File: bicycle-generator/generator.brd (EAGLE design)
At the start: 100 x 80 mm, 62 parts, among them IC1 MC34063AD, K1 ARK500/2, K2 ARK500/2, K3 ARK500/2, K4 ARK500/2, K5 ARK500/2, K6 HEAT_NPN, K7 ARK500/2, K8 ARK500/2, Q1 IRF3704S, Q2 IRF3704S, T1 BC807, T2 BC807, X1 CV_LED, X2 PWR_LED, X3 5V_SW, X4 5V_LED, X5 5V_OUT

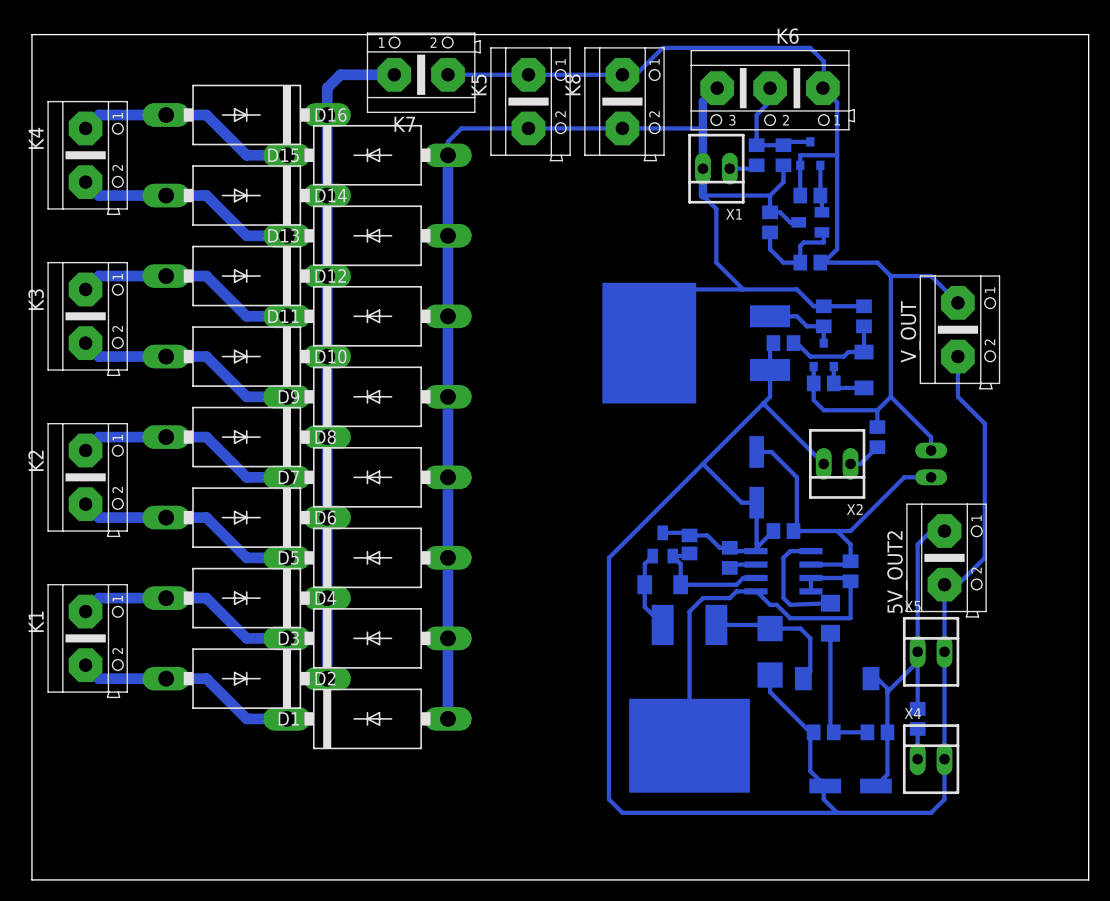
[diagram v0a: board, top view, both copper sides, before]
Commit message: Routed board.
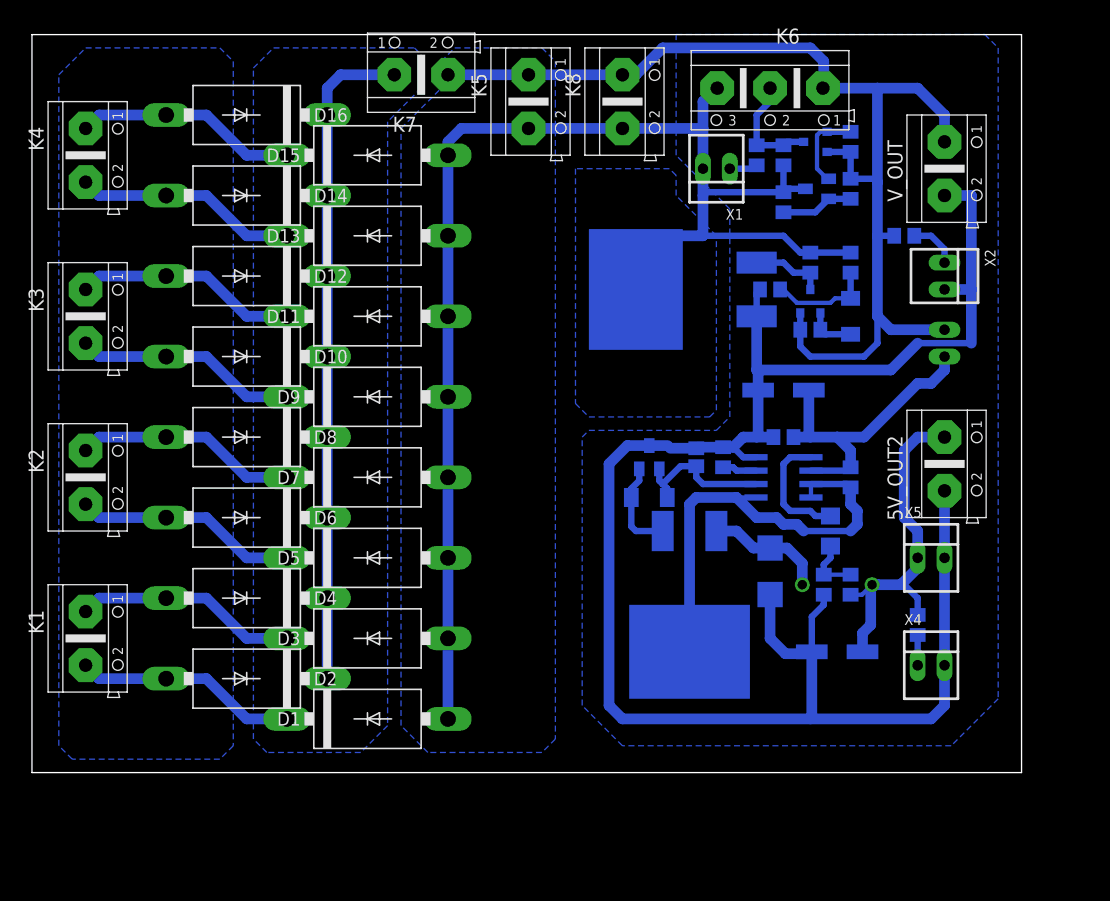
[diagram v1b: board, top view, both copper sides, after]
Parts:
- L1: device rcl:PIS2816 -> rcl:TJ3-U1
- moved X2 20.5 mm to (86.4, 57.1), turned to 270 degrees
- moved R10 19.2 mm to (82.5, 61.0), turned to 0 degrees
- moved V_OUT 15.3 mm to (86.4, 67.3)
- moved R11 14.2 mm to (77.5, 27.9), turned to 270 degrees
- moved R12 14.0 mm to (74.9, 27.9), turned to 90 degrees
- moved C3 12.8 mm to (76.2, 21.6)
- moved X3 11.5 mm to (86.4, 50.8)
- moved C1 9.55 mm to (65.4, 40.0)
- moved IC1 8.89 mm to (71.1, 38.1)
- moved L1 8.89 mm to (76.2, 27.9), turned to 180 degrees
- moved R13 8.89 mm to (77.5, 38.1)
- moved X4 8.89 mm to (85.1, 20.3)
- moved X5 8.89 mm to (85.1, 30.5)
- moved Q2 8.89 mm to (62.2, 24.1)
- moved R14 8.89 mm to (83.8, 24.1)
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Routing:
- net V-: track 139.7 -> 131.1 mm
- net N$11: track 12.7 -> 5.51 mm
- net N$27: track 38.4 -> 42.5 mm
- net N$3: track 4.60 -> 7.98 mm
- net V+: track 110.6 -> 107.5 mm
- net N$12: track 9.94 -> 6.88 mm
- net N$24: track 32.4 -> 30.0 mm
- net GND: track 174.5 -> 172.3 mm
- net N$19: track 13.5 -> 11.4 mm
- net N$28: track 12.1 -> 13.9 mm
- net N$23: track 3.20 -> 4.66 mm
- net N$15: track 7.53 -> 8.91 mm
- net +5V: track 35.2 -> 33.9 mm
- net N$16: track 2.61 -> 3.25 mm
- net N$7: track 11.1 -> 10.5 mm
- added copper zone on layer 16, net GND
- added copper zone on layer 16, net N$20
- added copper zone on layer 16, net N$25
- added copper zone on layer 16, net V-
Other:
- board size 100 x 80 mm -> 93.7 x 69.8 mm
